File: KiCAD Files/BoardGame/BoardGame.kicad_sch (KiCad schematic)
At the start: 0 parts

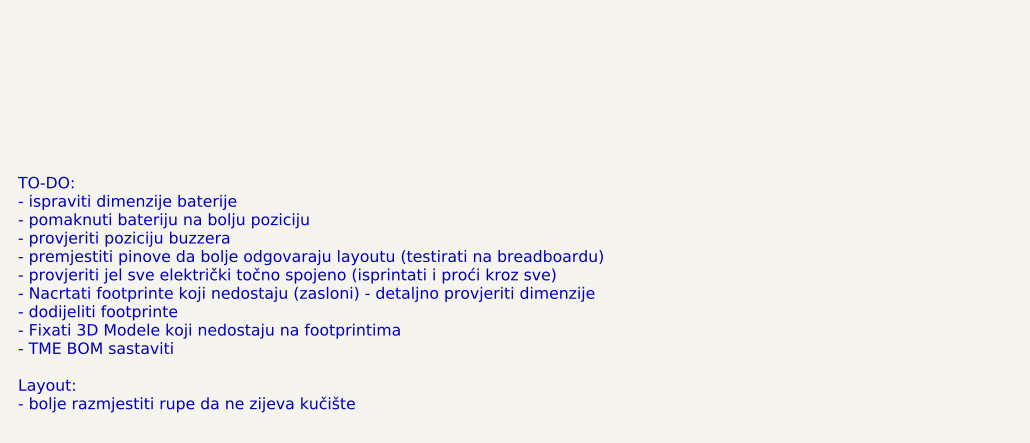
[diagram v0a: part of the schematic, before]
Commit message: update
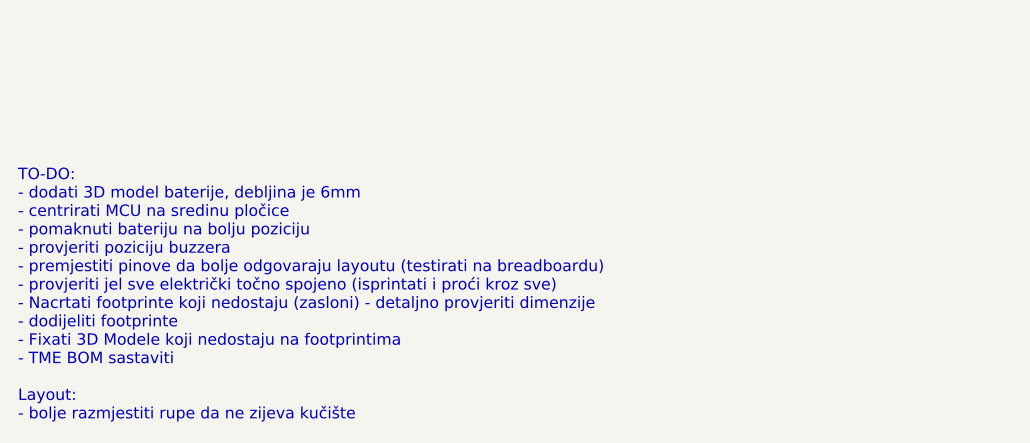
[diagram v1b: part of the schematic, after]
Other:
- note added: "TO-DO: - dodati 3D model baterije, debljina je 6mm - centrirati MCU na sredinu pločice - pomaknuti bateriju na bolju poziciju - provjeriti poziciju buzzera - premjestiti pinove da bolje odgovaraju layoutu (testirati na breadboardu) - provjeriti jel sve električki točno spojeno (isprintati i proći kroz sve) - Nacrtati footprinte koji nedostaju (zasloni) - detaljno provjeriti dimenzije - dodijeliti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"
- note removed: "TO-DO: - ispraviti dimenzije baterije - pomaknuti bateriju na bolju poziciju - provjeriti poziciju buzzera - premjestiti pinove da bolje odgovaraju layoutu (testirati na breadboardu) - provjeriti jel sve električki točno spojeno (isprintati i proći kroz sve) - Nacrtati footprinte koji nedostaju (zasloni) - detaljno provjeriti dimenzije - dodijeliti footprinte - Fixati 3D Modele koji nedostaju na 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"
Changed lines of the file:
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@@
 		)
 	)
-	(text "TO-DO:\n- ispraviti dimenzije baterije\n- pomaknuti bateriju na bolju poziciju\n- provjeriti poziciju buzzera\n- premjestiti pinove da bolje odgovaraju layoutu (testirati na breadboardu)\n- provjeriti jel sve električki točno spojeno (isprintati i proći kroz sve)\n- Nacrtati footprinte koji nedostaju (zasloni) - detaljno provjeriti dimenzije\n- dodijeliti footprinte\n- Fixati 3D Modele koji nedostaju na footprintima\n- TME BOM sastaviti\n\nLayout:\n- bolje razmjestiti rupe da ne zijeva kučište"
+	(text "TO-DO:\n- dodati 3D model baterije, debljina je 6mm\n- centrirati MCU na sredinu pločice\n- pomaknuti bateriju na bolju poziciju\n- provjeriti poziciju buzzera\n- premjestiti pinove da bolje odgovaraju layoutu (testirati na breadboardu)\n- provjeriti jel sve električki točno spojeno (isprintati i proći kroz sve)\n- Nacrtati footprinte koji nedostaju (zasloni) - detaljno provjeriti dimenzije\n- dodijeliti footprinte\n- Fixati 3D Modele koji nedostaju na footprintima\n- TME BOM sastaviti\n\nLayout:\n- bolje razmjestiti rupe da ne zijeva kučište"
 		(exclude_from_sim no)
 		(at 16.002 184.658 0)
